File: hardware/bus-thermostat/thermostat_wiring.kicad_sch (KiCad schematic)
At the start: 46 parts, among them Q2 2N7002, Q3 2N7002, Q4 2N7002, Q5 IRF540N, Q6 IRF540N, T1 PA2004NL, U2 UCC27714D, U3 PCA9557D

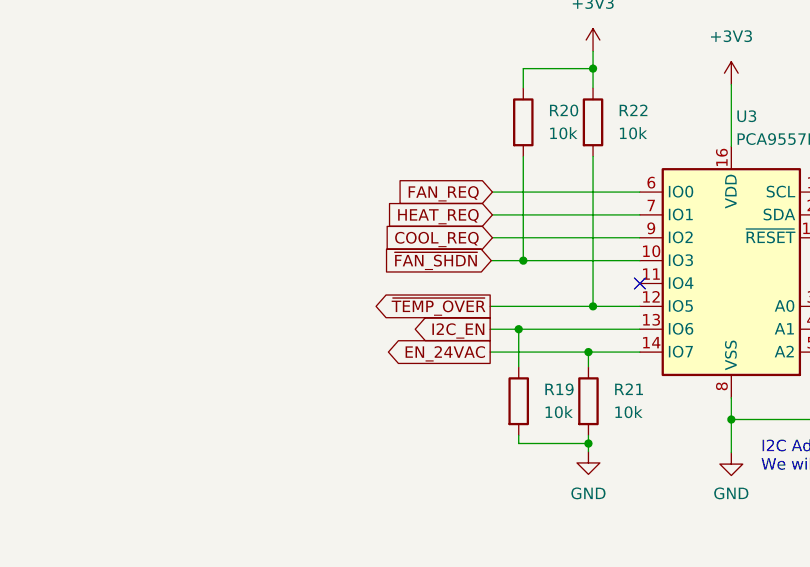
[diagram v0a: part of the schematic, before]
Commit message: Ooops forgot to save.
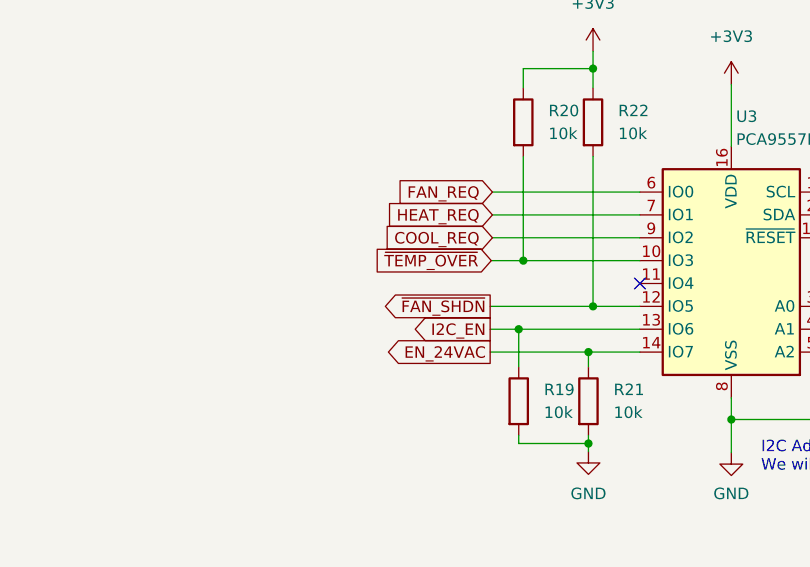
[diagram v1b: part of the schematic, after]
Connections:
- net ~{FAN_SHDN}: now also R22.2, U3.12 (IO5); no longer R20.2, U3.10 (IO3)
- net ~{TEMP_OVER}: now also R20.2, U3.10 (IO3); no longer R22.2, U3.12 (IO5)
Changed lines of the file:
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@@
     )
   )
-  (global_label "~{FAN_SHDN}" (shape input) (at 211.074 122.428 180) (fields_autoplaced)
+  (global_label "~{FAN_SHDN}" (shape output) (at 210.947 127.508 180) (fields_autoplaced)
     (effects (font (size 1.27 1.27)) (justify right))
-    (property "Intersheet References" "${INTERSHEET_REFS}" (id 0) (at 199.0452 122.3486 0)
+    (property "Intersheet References" "${INTERSHEET_REFS}" (id 0) (at 198.9182 127.4286 0)
       (effects (font (size 1.27 1.27)) (justify right) hide)
     )
@@
     )
   )
-  (global_label "~{TEMP_OVER}" (shape output) (at 210.947 127.508 180) (fields_autoplaced)
+  (global_label "~{TEMP_OVER}" (shape input) (at 211.074 122.428 180) (fields_autoplaced)
     (effects (font (size 1.27 1.27)) (justify right))
-    (property "Intersheet References" "${INTERSHEET_REFS}" (id 0) (at 197.8901 127.4286 0)
+    (property "Intersheet References" "${INTERSHEET_REFS}" (id 0) (at 198.0171 122.3486 0)
       (effects (font (size 1.27 1.27)) (justify right) hide)
     )
